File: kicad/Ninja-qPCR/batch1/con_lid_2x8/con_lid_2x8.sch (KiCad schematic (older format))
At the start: 8 parts, among them U1 Conn_02x05

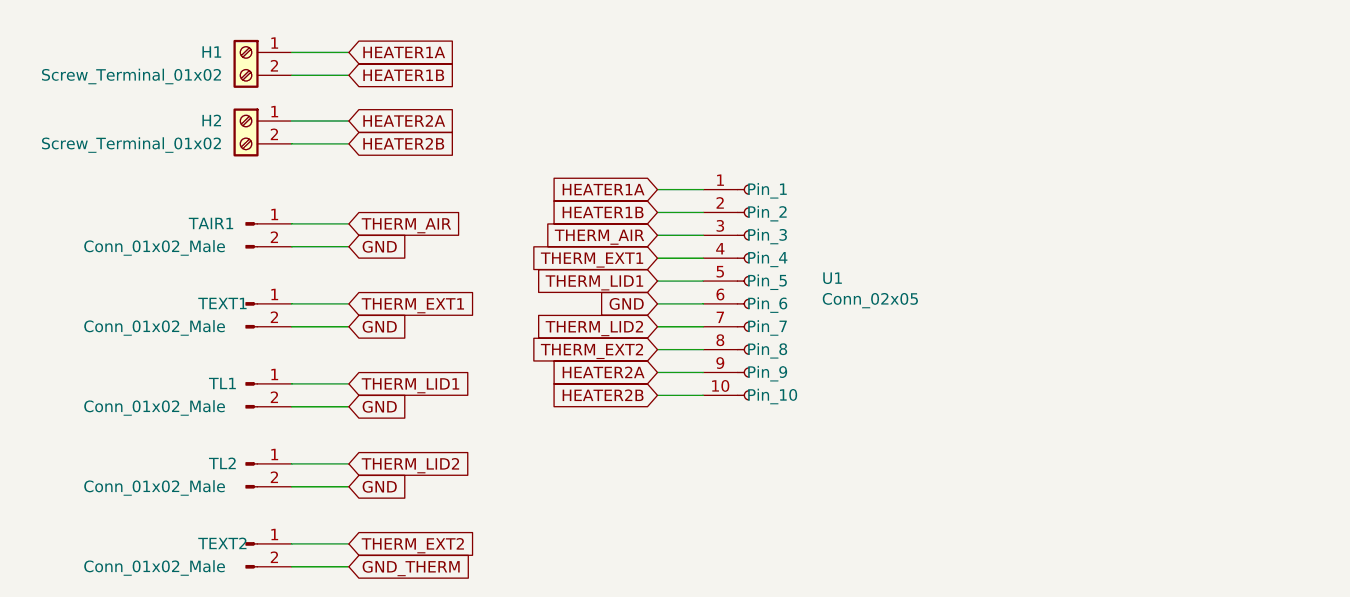
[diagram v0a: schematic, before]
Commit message: Add batch8 Photosensing and Main
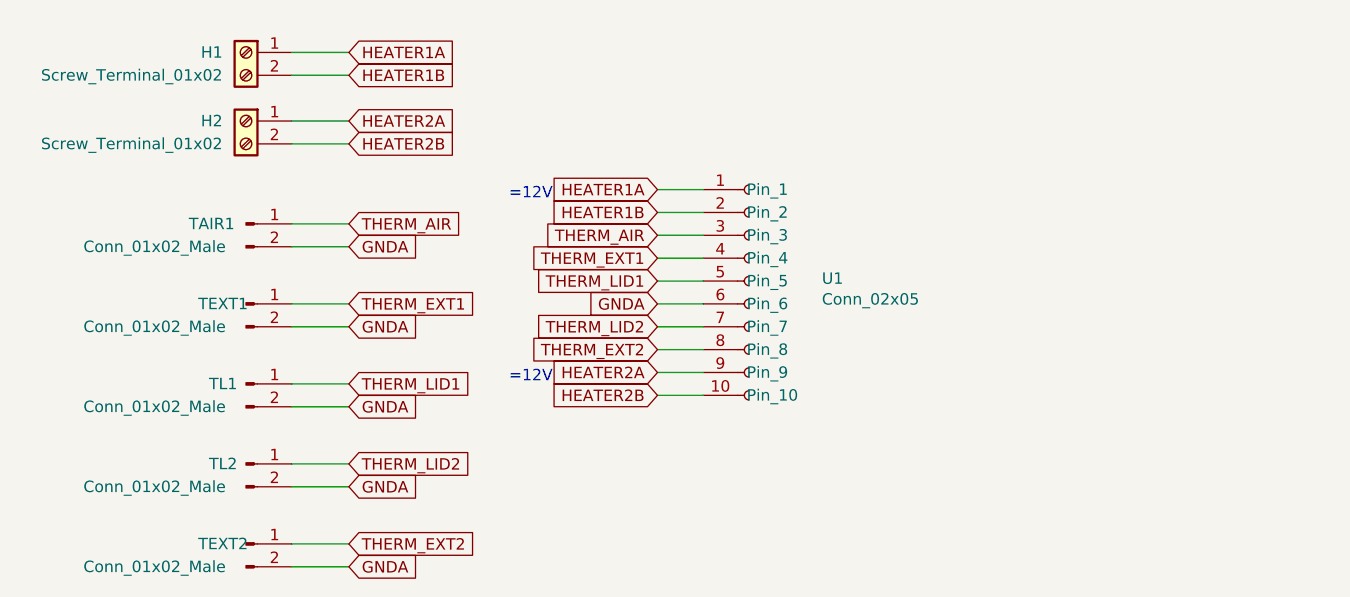
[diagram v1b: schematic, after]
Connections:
- net GND_THERM is gone; now on net GNDA: TEXT2.2 (Pin_2)
- net GND renamed GNDA
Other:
- note added: "=12V"
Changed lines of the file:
@@
 THERM_EXT2
 Text GLabel 3750 5050 2    50   Input ~ 0
-GND_THERM
+GNDA
 Wire Wire Line
 	3500 3550 3750 3550
@@
 	3750 5050 3500 5050
 Text GLabel 3750 4700 2    50   Input ~ 0
-GND
+GNDA
 Text GLabel 3750 4350 2    50   Input ~ 0
-GND
+GNDA
 Text GLabel 3750 4000 2    50   Input ~ 0
-GND
+GNDA
 Text GLabel 3750 3650 2    50   Input ~ 0
-GND
+GNDA
 Wire Wire Line
 	3500 3650 3750 3650
@@
 HEATER2B
 Text GLabel 5100 3900 0    50   Input ~ 0
-GND
+GNDA
 Text GLabel 5100 3600 0    50   Input ~ 0
 THERM_AIR
@@
 Wire Wire Line
 	5100 4200 5300 4200
+Text Notes 4450 3450 0    50   ~ 0
+=12V
+Text Notes 4450 4250 0    50   ~ 0
+=12V
 $EndSCHEMATC

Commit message: merge to one
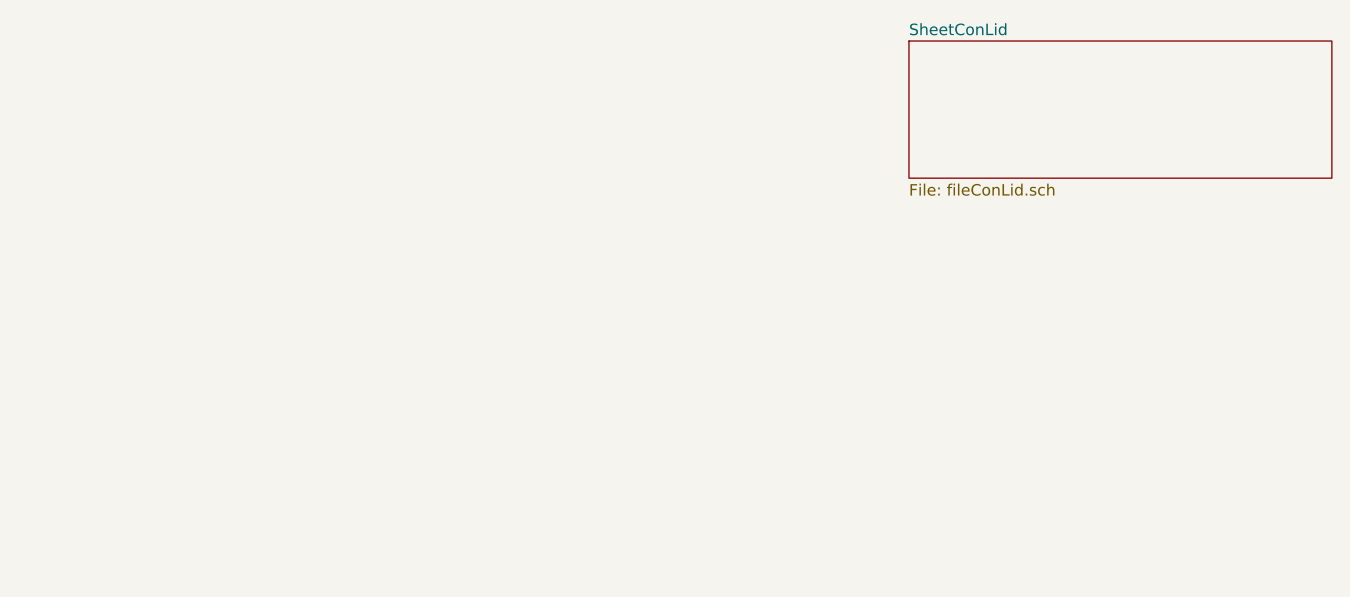
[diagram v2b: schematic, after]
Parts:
- removed H1, H2: Screw_Terminal_01x02, Ninja-qPCR:TB_SeeedOPL_320110028, symbol Connector:Screw_Terminal_01x02
- removed TAIR1, TEXT1, TEXT2, TL1, TL2: Conn_01x02_Male, Pin_Headers:Pin_Header_Angled_1x02_Pitch2.54mm, symbol Connector:Conn_01x02_Male
- removed U1: Conn_02x05, Pin_Headers:Pin_Header_Straight_2x05_Pitch2.54mm, symbol Ninja-qPCR:Conn_02x05
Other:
- note removed: "=12V"
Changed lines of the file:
@@
 $Descr A4 11693 8268
 encoding utf-8
-Sheet 1 1
+Sheet 1 2
 Title ""
 Date ""
@@
 Comment4 ""
 $EndDescr
-$Comp
-L Connector:Screw_Terminal_01x02 H1
-U 1 1 5F2B5266
-P 3300 2800
-F 0 "H1" H 3450 2800 50  0000 C CNN
-F 1 "Screw_Terminal_01x02" H 3800 2700 50  0000 C CNN
-F 2 "Ninja-qPCR:TB_SeeedOPL_320110028" H 3300 2800 50  0001 C CNN
-F 3 "~" H 3300 2800 50  0001 C CNN
-	1    3300 2800
-	-1   0    0    -1
-$EndComp
-$Comp
-L Connector:Conn_01x02_Male TEXT1
-U 1 1 5F2B7778
-P 3300 3900
-F 0 "TEXT1" H 3200 3900 50  0000 C CNN
-F 1 "Conn_01x02_Male" H 2900 3800 50  0000 C CNN
-F 2 "Pin_Headers:Pin_Header_Angled_1x02_Pitch2.54mm" H 3300 3900 50  0001 C CNN
-F 3 "~" H 3300 3900 50  0001 C CNN
-	1    3300 3900
-	1    0    0    -1
-$EndComp
-$Comp
-L Connector:Conn_01x02_Male TL1
-U 1 1 5F2BA46F
-P 3300 4250
-F 0 "TL1" H 3200 4250 50  0000 C CNN
-F 1 "Conn_01x02_Male" H 2900 4150 50  0000 C CNN
-F 2 "Pin_Headers:Pin_Header_Angled_1x02_Pitch2.54mm" H 3300 4250 50  0001 C CNN
-F 3 "~" H 3300 4250 50  0001 C CNN
-	1    3300 4250
-	1    0    0    -1
-$EndComp
-$Comp
-L Connector:Conn_01x02_Male TL2
-U 1 1 5F2BA479
-P 3300 4600
-F 0 "TL2" H 3200 4600 50  0000 C CNN
-F 1 "Conn_01x02_Male" H 2900 4500 50  0000 C CNN
-F 2 "Pin_Headers:Pin_Header_Angled_1x02_Pitch2.54mm" H 3300 4600 50  0001 C CNN
-F 3 "~" H 3300 4600 50  0001 C CNN
-	1    3300 4600
-	1    0    0    -1
-$EndComp
-$Comp
-L Connector:Conn_01x02_Male TEXT2
-U 1 1 5F2BC0F4
-P 3300 4950
-F 0 "TEXT2" H 3200 4950 50  0000 C CNN
-F 1 "Conn_01x02_Male" H 2900 4850 50  0000 C CNN
-F 2 "Pin_Headers:Pin_Header_Angled_1x02_Pitch2.54mm" H 3300 4950 50  0001 C CNN
-F 3 "~" H 3300 4950 50  0001 C CNN
-	1    3300 4950
-	1    0    0    -1
-$EndComp
-$Comp
-L Ninja-qPCR:Conn_02x05 U1
-U 1 1 5F2BEF9C
-P 5500 3400
-F 0 "U1" H 5819 3011 50  0000 L CNN
-F 1 "Conn_02x05" H 5819 2920 50  0000 L CNN
-F 2 "Pin_Headers:Pin_Header_Straight_2x05_Pitch2.54mm" H 5300 3500 50  0001 C CNN
-F 3 "" H 5300 3500 50  0001 C CNN
-	1    5500 3400
-	1    0    0    -1
-$EndComp
-Text GLabel 3750 2800 2    50   Input ~ 0
-HEATER1A
-Text GLabel 3750 2900 2    50   Input ~ 0
-HEATER1B
-Text GLabel 3750 3100 2    50   Input ~ 0
-HEATER2A
-Text GLabel 3750 3200 2    50   Input ~ 0
-HEATER2B
-Text GLabel 3750 3900 2    50   Input ~ 0
-THERM_EXT1
-Text GLabel 3750 4250 2    50   Input ~ 0
-THERM_LID1
-Text GLabel 3750 3550 2    50   Input ~ 0
-THERM_AIR
-Text GLabel 3750 4600 2    50   Input ~ 0
-THERM_LID2
-Text GLabel 3750 4950 2    50   Input ~ 0
-THERM_EXT2
-Text GLabel 3750 5050 2    50   Input ~ 0
-GNDA
-Wire Wire Line
-	3500 3550 3750 3550
-Wire Wire Line
-	3750 3900 3500 3900
-Wire Wire Line
-	3750 2800 3500 2800
-Wire Wire Line
-	3750 2900 3500 2900
-Wire Wire Line
-	3750 3100 3500 3100
-Wire Wire Line
-	3750 3200 3500 3200
-Wire Wire Line
-	3750 4250 3500 4250
-Wire Wire Line
-	3750 4600 3500 4600
-Wire Wire Line
-	3750 4950 3500 4950
-Wire Wire Line
-	3750 5050 3500 5050
-Text GLabel 3750 4700 2    50   Input ~ 0
-GNDA
-Text GLabel 3750 4350 2    50   Input ~ 0
-GNDA
-Text GLabel 3750 4000 2    50   Input ~ 0
-GNDA
-Text GLabel 3750 3650 2    50   Input ~ 0
-GNDA
-Wire Wire Line
-	3500 3650 3750 3650
-Wire Wire Line
-	3500 4000 3750 4000
-Wire Wire Line
-	3500 4350 3750 4350
-Wire Wire Line
-	3500 4700 3750 4700
-Text GLabel 5100 3400 0    50   Input ~ 0
-HEATER1A
-Text GLabel 5100 3500 0    50   Input ~ 0
-HEATER1B
-Text GLabel 5100 4200 0    50   Input ~ 0
-HEATER2A
-Text GLabel 5100 4300 0    50   Input ~ 0
-HEATER2B
-Text GLabel 5100 3900 0    50   Input ~ 0
-GNDA
-Text GLabel 5100 3600 0    50   Input ~ 0
-THERM_AIR
-Text GLabel 5100 3700 0    50   Input ~ 0
-THERM_EXT1
-Text GLabel 5100 3800 0    50   Input ~ 0
-THERM_LID1
-Text GLabel 5100 4000 0    50   Input ~ 0
-THERM_LID2
-Text GLabel 5100 4100 0    50   Input ~ 0
-THERM_EXT2
-Wire Wire Line
-	5100 3400 5300 3400
-Wire Wire Line
-	5100 3600 5300 3600
-Wire Wire Line
-	5100 3700 5300 3700
-Wire Wire Line
-	5100 3800 5300 3800
-Wire Wire Line
-	5100 3900 5300 3900
-Wire Wire Line
-	5100 4000 5300 4000
-Wire Wire Line
-	5100 4100 5300 4100
-Wire Wire Line
-	5100 4300 5300 4300
-$Comp
-L Connector:Screw_Terminal_01x02 H2
-U 1 1 5F2B5A56
-P 3300 3100
-F 0 "H2" H 3450 3100 50  0000 C CNN
-F 1 "Screw_Terminal_01x02" H 3800 3000 50  0000 C CNN
-F 2 "Ninja-qPCR:TB_SeeedOPL_320110028" H 3300 3100 50  0001 C CNN
-F 3 "~" H 3300 3100 50  0001 C CNN
-	1    3300 3100
-	-1   0    0    -1
-$EndComp
-$Comp
-L Connector:Conn_01x02_Male TAIR1
-U 1 1 5F2B6313
-P 3300 3550
-F 0 "TAIR1" H 3150 3550 50  0000 C CNN
-F 1 "Conn_01x02_Male" H 2900 3450 50  0000 C CNN
-F 2 "Pin_Headers:Pin_Header_Angled_1x02_Pitch2.54mm" H 3300 3550 50  0001 C CNN
-F 3 "~" H 3300 3550 50  0001 C CNN
-	1    3300 3550
-	1    0    0    -1
-$EndComp
-Wire Wire Line
-	5100 3500 5300 3500
-Wire Wire Line
-	5100 4200 5300 4200
-Text Notes 4450 3450 0    50   ~ 0
-=12V
-Text Notes 4450 4250 0    50   ~ 0
-=12V
+$Sheet
+S 6200 2750 1850 600
+U 60B5A248
+F0 "SheetConLid" 50
+F1 "fileConLid.sch" 50
+$EndSheet
 $EndSCHEMATC
